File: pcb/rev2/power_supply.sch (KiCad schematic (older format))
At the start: 48 parts, among them IC3 LV52204MUTBG, IC4 LM26480, IC5 TPS61040

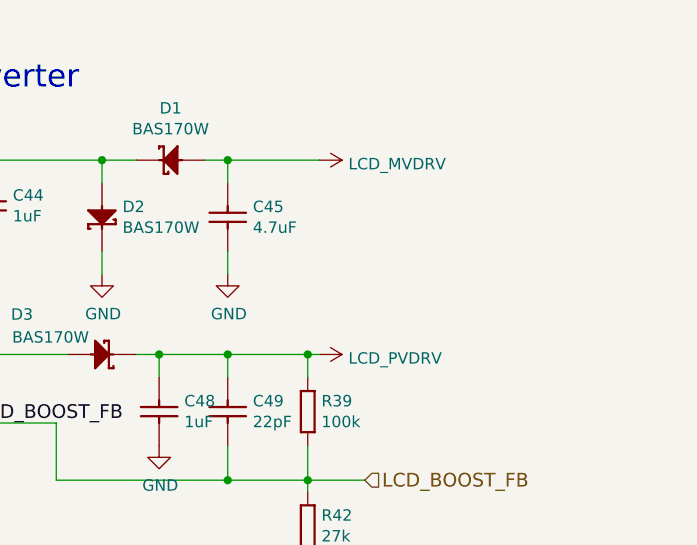
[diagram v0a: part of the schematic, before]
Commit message: pcb wip
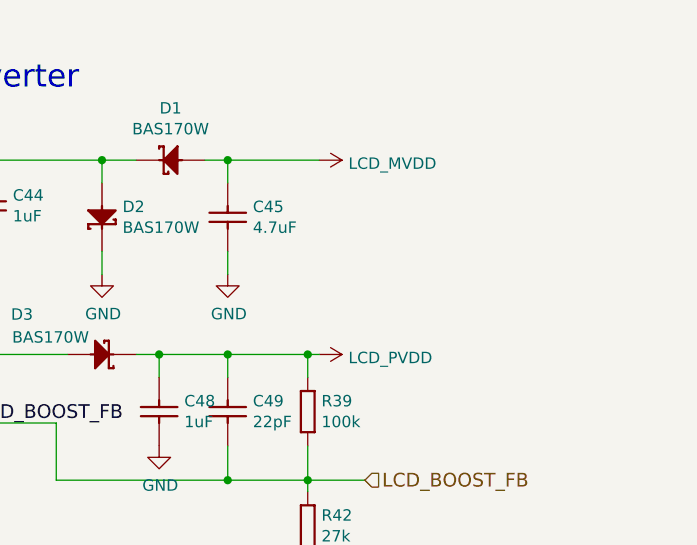
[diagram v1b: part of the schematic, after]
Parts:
- C41, C42, C43, C44, C45, C47, C48, C49, C51, C53, C55, C56, C57, C62, C63, C74, C78: footprint CAPC1608X87N -> Capacitors SMD:CAPC1608X87N
- C46, C50, C54, C58: footprint CAPC2012X135N -> Capacitors SMD:CAPC2012X135N
- C60, C61: footprint CAPMP3528X210N -> Capacitors SMD:CAPMP3528X210N
- D1, D2, D3, D4: footprint SOD3715X145N -> ICs And Semiconductors SMD:SOD3715X145N
- IC3: footprint (none) -> dsi_shield:UDFN6_2X2_065P
- IC4: footprint (none) -> ICs And Semiconductors SMD:QFN50P400X400X80-25N-S230
- IC5: footprint (none) -> ICs And Semiconductors SMD:SOT65P210X110-5N
- L2, L3, L4, L5: footprint (none) -> dsi_shield:IND_PANASONIC_ELLVEG
- R35, R36, R37, R38, R39, R40, R41, R42, R43, R44, R45, R46, R47, R53: footprint RESC1608X55N -> Resistors SMD:RESC1608X55N
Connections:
- net LCD_MVDRV renamed LCD_MVDD
- net LCD_PVDRV renamed LCD_PVDD
